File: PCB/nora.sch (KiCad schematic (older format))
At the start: 231 parts, among them J1 USB_C_Receptacle_USB2.0, J2 Conn_01x04, J3 Conn_01x02, J5 Conn_02x03_Odd_Even, U1 ATmega32U4-MU, U2 24LC64, U4 Pico, Y1 16MHz

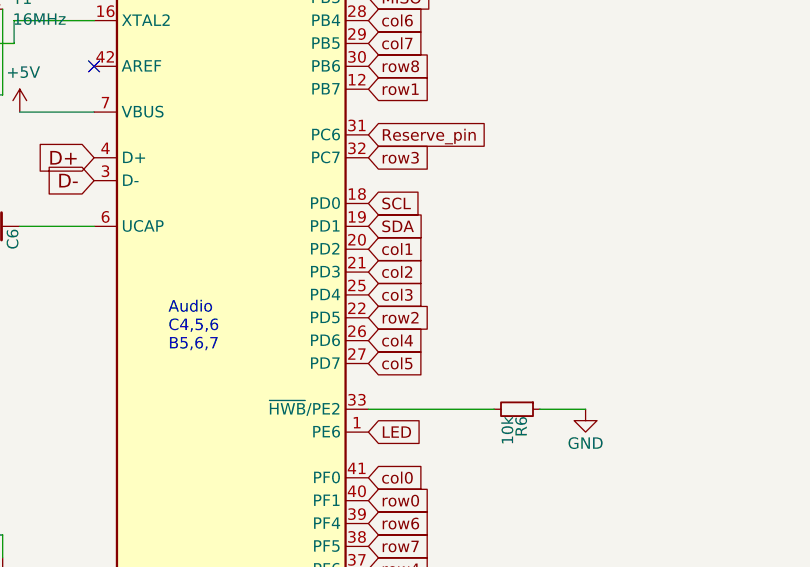
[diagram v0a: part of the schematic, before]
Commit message: WIP 配線
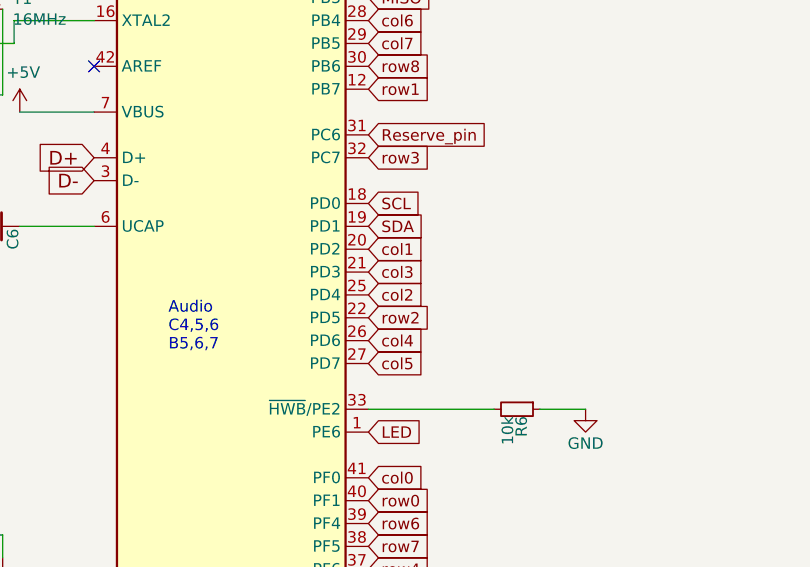
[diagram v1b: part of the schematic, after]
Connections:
- net col2: now also U1.25 (PD4); no longer U1.21 (PD3)
- net col3: now also U1.21 (PD3); no longer U1.25 (PD4)
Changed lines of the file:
@@
 Text GLabel 15325 3275 2    50   Input ~ 0
 col1
-Text GLabel 15325 3475 2    50   Input ~ 0
+Text GLabel 15325 3375 2    50   Input ~ 0
 col3
 Text GLabel 15325 3775 2    50   Input ~ 0
@@
 Text GLabel 15325 1975 2    50   Input ~ 0
 SCK
-Text GLabel 15325 3375 2    50   Input ~ 0
+Text GLabel 15325 3475 2    50   Input ~ 0
 col2
 Text GLabel 15325 3575 2    50   Input ~ 0
